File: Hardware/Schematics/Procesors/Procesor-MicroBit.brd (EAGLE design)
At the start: 59 x 44 mm, 2 parts

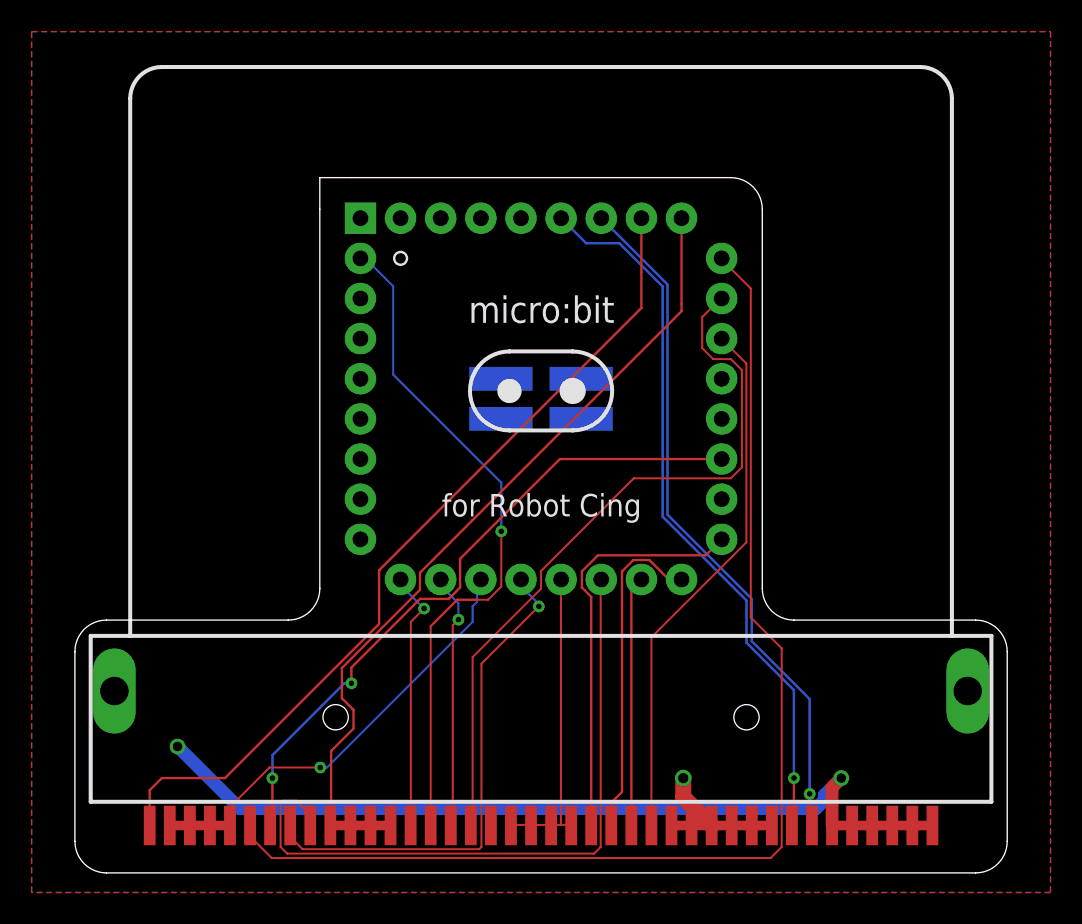
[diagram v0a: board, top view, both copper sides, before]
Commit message: microBit board
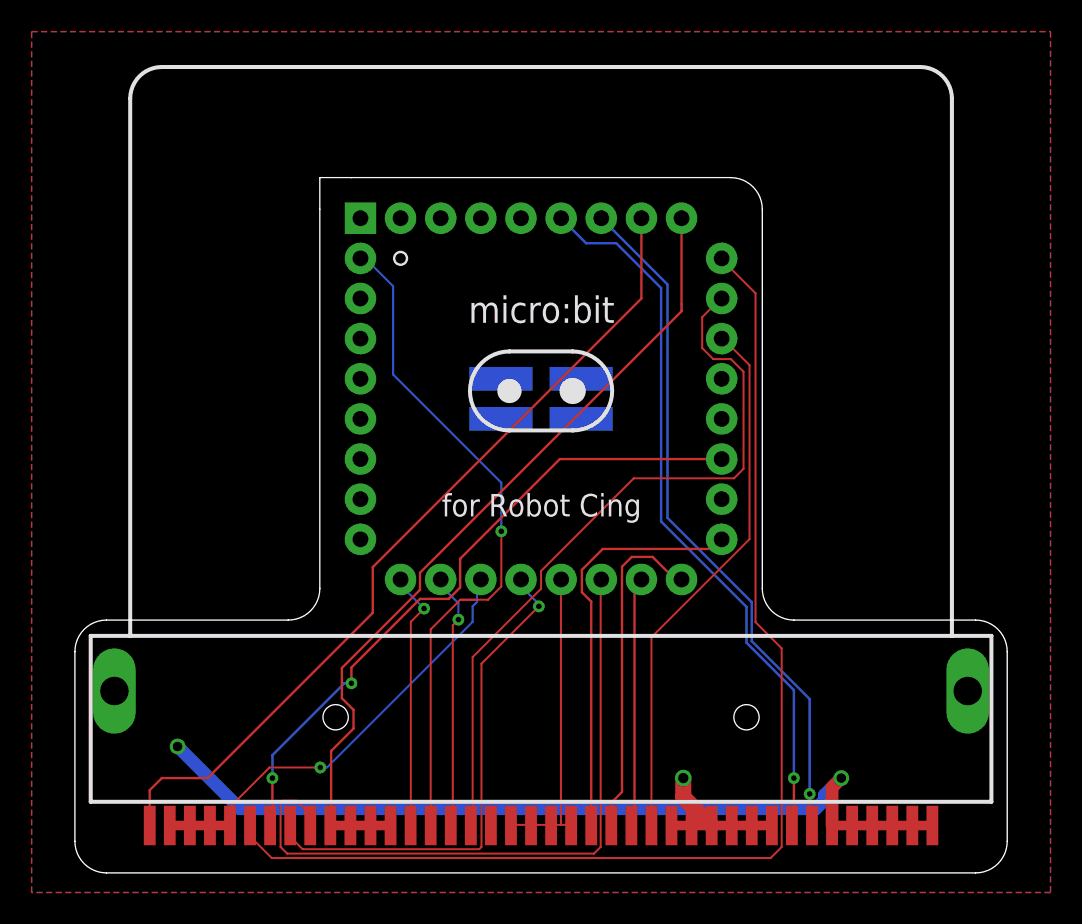
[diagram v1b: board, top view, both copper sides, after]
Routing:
- net A3: track 53.7 -> 53.0 mm

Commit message: microBit board
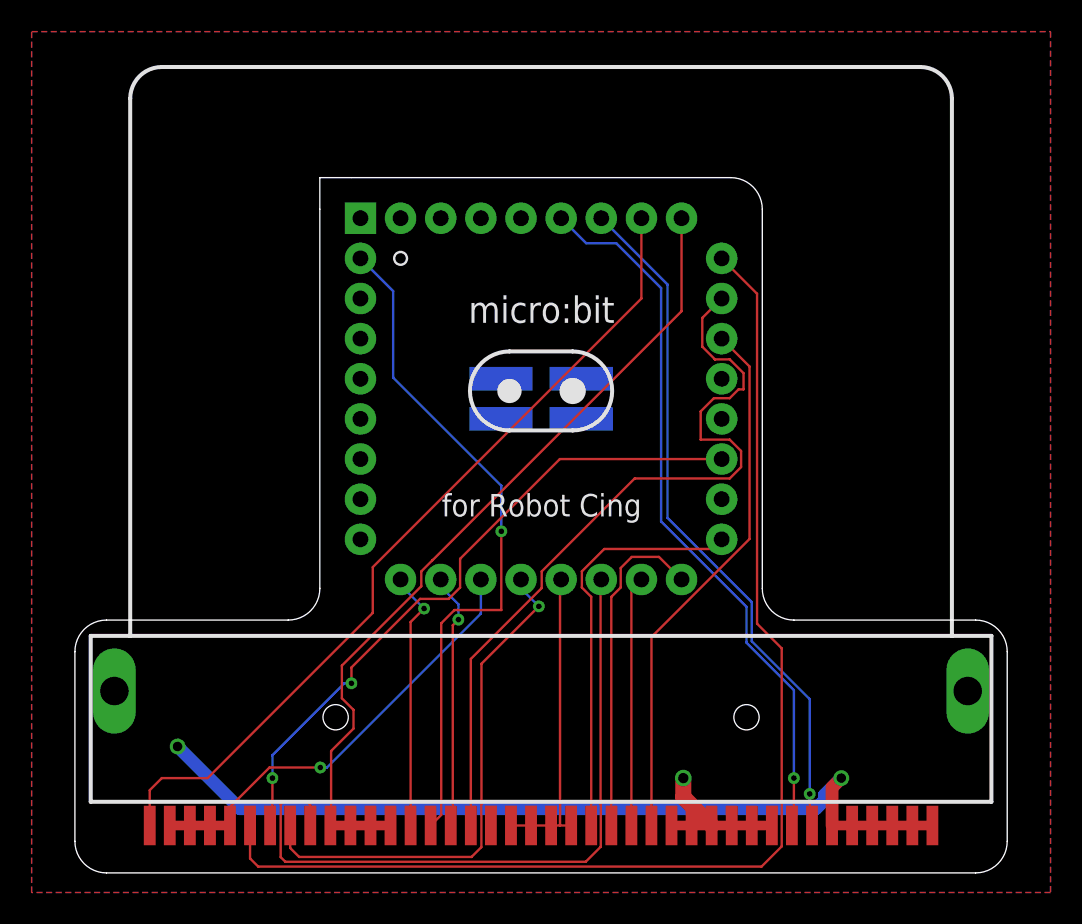
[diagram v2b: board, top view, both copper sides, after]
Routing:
- net A0: track 46.5 -> 50.1 mm
- net A1: track 74.0 -> 75.3 mm
- net D10: track 43.3 -> 44.4 mm
- net D8: track 32.1 -> 32.9 mm
- net D3: track 42.6 -> 43.2 mm
